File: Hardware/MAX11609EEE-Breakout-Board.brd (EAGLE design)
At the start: 160 x 100 mm, 0 parts

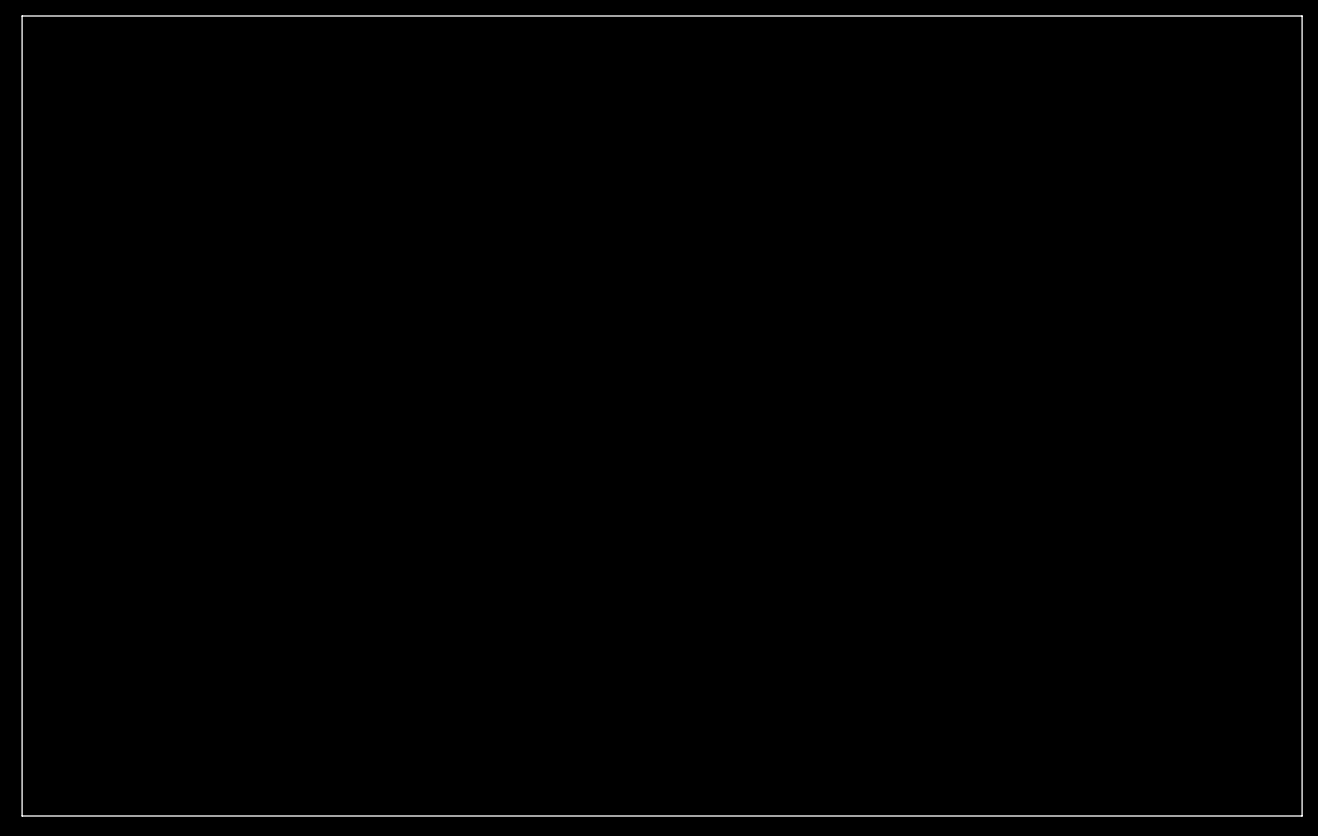
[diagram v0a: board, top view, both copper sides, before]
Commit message: These are the files that were sent to OSHPARK
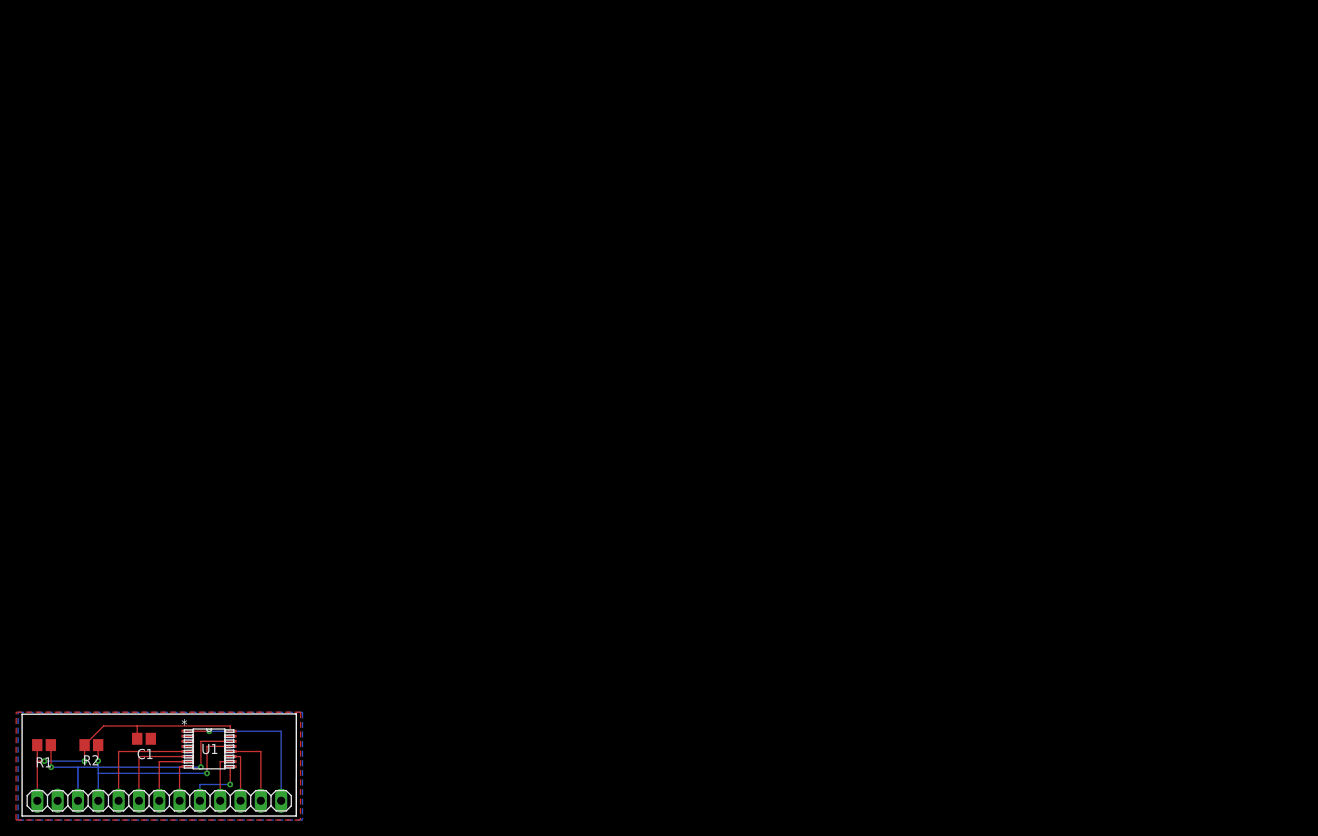
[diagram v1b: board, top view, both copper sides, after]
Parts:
- added C1: 0.1uF, resistor:C0805
- added JP3: (no value), pinhead:1X13
- added R1, R2: 4.7k, resistor:R0805
- added U1: MAX11609EEE+, MAX11609EEE:21-0055H_16
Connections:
- new net AIN0: JP3.5, U1.5
- new net AIN1: JP3.6, U1.6
- new net AIN2: JP3.7, U1.7
- new net AIN3: JP3.8, U1.8
- new net AIN4: JP3.9, U1.9
- new net AIN5: JP3.10, U1.10
- new net AIN6: JP3.11, U1.11
- new net AIN7: JP3.12, U1.12
- new net GND: C1.2, JP3.2, U1.15
- new net REF: JP3.13, U1.1
- new net SCL: JP3.4, R2.1, U1.13
- new net SDA: JP3.3, R1.1, U1.14
- new net VDD: C1.1, JP3.1, R1.2, R2.2, U1.16
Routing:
- net VDD: track 0.00 -> 36.3 mm, vias 0 -> 2
- net SDA: track 0.00 -> 32.6 mm, vias 0 -> 2
- net SCL: track 0.00 -> 26.8 mm, vias 0 -> 2
- net REF: track 0.00 -> 20.4 mm, vias 0 -> 1
- net AIN0: track 0.00 -> 14.8 mm
- net AIN1: track 0.00 -> 11.6 mm
- net AIN7: track 0.00 -> 9.98 mm
- net AIN2: track 0.00 -> 8.46 mm
- net AIN4: track 0.00 -> 8.04 mm, vias 0 -> 1
- net AIN6: track 0.00 -> 6.81 mm
- net AIN5: track 0.00 -> 6.15 mm
- net AIN3: track 0.00 -> 5.28 mm
- added copper zone on layer 1, net GND
- added copper zone on layer 16, net GND
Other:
- board size 160 x 100 mm -> 34.3 x 12.8 mm
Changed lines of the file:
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@@
 <setting verticaltext="up"/>
 </settings>
-<grid distance="0.05" unitdist="inch" unit="inch" style="lines" multiple="1" display="no" altdistance="0.025" altunitdist="inch" altunit="inch"/>
+<grid distance="10" unitdist="mil" unit="mil" style="lines" multiple="1" display="no" altdistance="0.01" altunitdist="mil" altunit="mil"/>
 <layers>
 <layer number="1" name="Top" color="4" fill="1" visible="yes" active="yes"/>
@@
 <board>
 <plain>
-<wire x1="0" y1="0" x2="160" y2="0" width="0" layer="20"/>
-<wire x1="160" y1="0" x2="160" y2="100" width="0" layer="20"/>
-<wire x1="160" y1="100" x2="0" y2="100" width="0" layer="20"/>
-<wire x1="0" y1="100" x2="0" y2="0" width="0" layer="20"/>
+<wire x1="0" y1="0" x2="34.27" y2="0" width="0" layer="20"/>
+<wire x1="34.27" y1="0" x2="34.27508125" y2="12.756078125" width="0" layer="20"/>
+<wire x1="34.27508125" y1="12.756078125" x2="0" y2="12.7256" width="0" layer="20"/>
+<wire x1="0" y1="12.7256" x2="0" y2="0" width="0" layer="20"/>
+<dimension x1="0" y1="0" x2="34.27" y2="0" x3="17.135" y3="-3.302" textsize="1.778" layer="20" dtype="horizontal" unit="inch"/>
+<dimension x1="0" y1="12.7256" x2="0" y2="0" x3="-3.302" y3="6.3628" textsize="1.778" layer="20" dtype="vertical" unit="inch"/>
 </plain>
 <attributes>
@@
 </autorouter>
 <elements>
+<element name="U1" library="MAX11609EEE" package="21-0055H_16" value="MAX11609EEE+" x="23.368" y="8.382" smashed="yes">
+<attribute name="VENDOR" value="Maxim" x="23.368" y="8.382" size="1.778" layer="27" display="off"/>
+<attribute name="MANUFACTURER_NAME" value="Maxim" x="23.368" y="8.382" size="1.778" layer="27" display="off"/>
+<attribute name="MANUFACTURER_PART_NUMBER" value="MAX11609EEE+" x="23.368" y="8.382" size="1.778" layer="27" display="off"/>
+<attribute name="NAME" x="22.4028" y="7.747" size="1.27" layer="25" ratio="6" rot="SR0"/>
+</element>
+<element name="R1" library="resistor" package="R0805" value="4.7k" x="2.7432" y="8.8646" smashed="yes" rot="R180">
+<attribute name="NAME" x="3.7592" y="7.3406" size="1.27" layer="25" rot="R180"/>
+</element>
+<element name="R2" library="resistor" package="R0805" value="4.7k" x="8.6614" y="8.8646" smashed="yes" rot="R180">
+<attribute name="NAME" x="9.6774" y="7.5946" size="1.27" layer="25" rot="R180"/>
+</element>
+<element name="C1" library="resistor" package="C0805" value="0.1uF" x="15.24" y="9.652" smashed="yes">
+<attribute name="NAME" x="14.351" y="7.112" size="1.27" layer="25"/>
+</element>
+<element name="JP3" library="pinhead" package="1X13" value="" x="17.145" y="1.905" smashed="yes">
+<attribute name="VALUE" x="0.635" y="-1.27" size="1.27" layer="27"/>
+</element>
 </elements>
 <signals>
+<signal name="VDD">
+<contactref element="R1" pad="2"/>
+<contactref element="R2" pad="2"/>
+<contactref element="U1" pad="16"/>
+<contactref element="C1" pad="1"/>
+<contactref element="JP3" pad="1"/>
+<via x="2.794" y="6.858" extent="1-16" drill="0.3302"/>
+<wire x1="2.794" y1="6.858" x2="7.7978" y2="6.858" width="0.1524" layer="16"/>
+<via x="7.7978" y="6.858" extent="1-16" drill="0.3302"/>
+<wire x1="7.7978" y1="6.858" x2="7.8114" y2="7.5574" width="0.1524" layer="1"/>
+<wire x1="7.8114" y1="7.5574" x2="7.8114" y2="8.8646" width="0.1524" layer="1"/>
+<wire x1="14.39" y1="9.652" x2="14.39" y2="11.2522" width="0.1524" layer="1"/>
+<wire x1="14.39" y1="11.2522" x2="26.035" y2="11.2522" width="0.1524" layer="1"/>
+<wire x1="26.035" y1="11.2522" x2="26.0223" y2="10.6045" width="0.1524" layer="1"/>
+<wire x1="7.8114" y1="8.8646" x2="10.199" y2="11.2522" width="0.1524" layer="1"/>
+<wire x1="10.199" y1="11.2522" x2="14.39" y2="11.2522" width="0.1524" layer="1"/>
+<wire x1="1.905" y1="1.905" x2="1.896603125" y2="6.857340625" width="0.1524" layer="1"/>
+<wire x1="1.896603125" y1="6.857340625" x2="1.8932" y2="8.8646" width="0.1524" layer="1"/>
+<wire x1="2.794" y1="6.858" x2="1.896603125" y2="6.857340625" width="0.1524" layer="1"/>
+</signal>
+<signal name="SDA">
+<contactref element="U1" pad="14"/>
+<contactref element="R1" pad="1"/>
+<contactref element="JP3" pad="3"/>
+<wire x1="6.985" y1="1.905" x2="6.985" y2="6.096" width="0.1524" layer="16"/>
+<wire x1="6.985" y1="6.096" x2="22.352" y2="6.096" width="0.1524" layer="16"/>
+<via x="22.352" y="6.096" extent="1-16" drill="0.3302"/>
+<wire x1="22.352" y1="6.096" x2="22.352" y2="9.3345" width="0.1524" layer="1"/>
+<wire x1="22.352" y1="9.3345" x2="26.0223" y2="9.3345" width="0.1524" layer="1"/>
+<wire x1="3.5932" y1="8.8646" x2="3.6322" y2="6.096" width="0.1524" layer="1"/>
+<via x="3.6322" y="6.096" extent="1-16" drill="0.3302"/>
+<wire x1="3.6322" y1="6.096" x2="6.985" y2="6.096" width="0.1524" layer="16"/>
+</signal>
+<signal name="SCL">
+<contactref element="U1" pad="13"/>
+<contactref element="R2" pad="1"/>
+<contactref element="JP3" pad="4"/>
+<wire x1="9.525" y1="1.905" x2="9.525" y2="5.334" width="0.1524" layer="16"/>
+<wire x1="9.525" y1="5.334" x2="23.114" y2="5.334" width="0.1524" layer="16"/>
+<via x="23.114" y="5.334" extent="1-16" drill="0.3302"/>
+<wire x1="23.114" y1="5.334" x2="23.114" y2="8.6995" width="0.1524" layer="1"/>
+<wire x1="23.114" y1="8.6995" x2="26.0223" y2="8.6995" width="0.1524" layer="1"/>
+<wire x1="9.5114" y1="8.8646" x2="9.4996" y2="6.8834" width="0.1524" layer="1"/>
+<via x="9.4996" y="6.8834" extent="1-16" drill="0.3302"/>
+<wire x1="9.4996" y1="6.8834" x2="9.525" y2="5.334" width="0.1524" layer="16"/>
+</signal>
+<signal name="AIN7">
+<contactref element="U1" pad="12"/>
+<contactref element="JP3" pad="12"/>
+<wire x1="26.0223" y1="8.0645" x2="29.845" y2="8.0645" width="0.1524" layer="1"/>
+<wire x1="29.845" y1="8.0645" x2="29.845" y2="1.905" width="0.1524" layer="1"/>
+</signal>
+<signal name="AIN6">
+<contactref element="U1" pad="11"/>
+<contactref element="JP3" pad="11"/>
+<wire x1="26.0223" y1="7.4295" x2="27.305" y2="7.4295" width="0.1524" layer="1"/>
+<wire x1="27.305" y1="7.4295" x2="27.305" y2="1.905" width="0.1524" layer="1"/>
+</signal>
+<signal name="AIN5">
+<contactref element="U1" pad="10"/>
+<contactref element="JP3" pad="10"/>
+<wire x1="26.0223" y1="6.7945" x2="24.765" y2="6.7945" width="0.1524" layer="1"/>
+<wire x1="24.765" y1="6.7945" x2="24.765" y2="1.905" width="0.1524" layer="1"/>
+</signal>
+<signal name="AIN4">
+<contactref element="U1" pad="9"/>
+<contactref element="JP3" pad="9"/>
+<wire x1="26.0223" y1="6.1595" x2="26.0096" y2="3.937" width="0.1524" layer="1"/>
+<via x="26.0096" y="3.937" extent="1-16" drill="0.3302"/>
+<wire x1="26.0096" y1="3.937" x2="22.225" y2="3.937" width="0.1524" layer="16"/>
+<wire x1="22.225" y1="3.937" x2="22.225" y2="1.905" width="0.1524" layer="16"/>
+</signal>
+<signal name="AIN0">
+<contactref element="U1" pad="5"/>
+<contactref element="JP3" pad="5"/>
+<wire x1="20.7137" y1="8.0645" x2="12.065" y2="8.0645" width="0.1524" layer="1"/>
+<wire x1="12.065" y1="8.0645" x2="12.065" y2="1.905" width="0.1524" layer="1"/>
+</signal>
+<signal name="AIN1">
+<contactref element="U1" pad="6"/>
+<contactref element="JP3" pad="6"/>
+<wire x1="20.7137" y1="7.4295" x2="14.605" y2="7.4295" width="0.1524" layer="1"/>
+<wire x1="14.605" y1="7.4295" x2="14.605" y2="1.905" width="0.1524" layer="1"/>
+</signal>
+<signal name="AIN2">
+<contactref element="U1" pad="7"/>
+<contactref element="JP3" pad="7"/>
+<wire x1="20.7137" y1="6.7945" x2="17.145" y2="6.7945" width="0.1524" layer="1"/>
+<wire x1="17.145" y1="6.7945" x2="17.145" y2="1.905" width="0.1524" layer="1"/>
+</signal>
+<signal name="AIN3">
+<contactref element="U1" pad="8"/>
+<contactref element="JP3" pad="8"/>
+<wire x1="20.7137" y1="6.1595" x2="19.685" y2="6.1595" width="0.1524" layer="1"/>
+<wire x1="19.685" y1="6.1595" x2="19.685" y2="1.905" width="0.1524" layer="1"/>
+</signal>
+<signal name="REF">
+<contactref element="U1" pad="1"/>
+<contactref element="JP3" pad="13"/>
+<wire x1="20.7137" y1="10.6045" x2="23.3934" y2="10.5918" width="0.1524" layer="1"/>
+<via x="23.3934" y="10.5918" extent="1-16" drill="0.3302"/>
+<wire x1="23.3934" y1="10.5918" x2="32.385" y2="10.5918" width="0.1524" layer="16"/>
+<wire x1="32.385" y1="10.5918" x2="32.385" y2="1.905" width="0.1524" layer="16"/>
+</signal>
+<signal name="GND">
+<contactref element="JP3" pad="2"/>
+<contactref element="U1" pad="15"/>
+<contactref element="C1" pad="2"/>
+<polygon width="0.1524" layer="1">
+<vertex x="-0.7366" y="12.9794"/>
+<vertex x="34.8234" y="12.9794"/>
+<vertex x="34.798" y="-0.508"/>
+<vertex x="-0.762" y="-0.508"/>
+</polygon>
+<polygon width="0.1524" layer="16">
+<vertex x="-0.508" y="12.954"/>
+<vertex x="35.052" y="12.954"/>
+<vertex x="35.052" y="-0.508"/>
+<vertex x="-0.508" y="-0.508"/>
+</polygon>
+</signal>
 </signals>
 </board>
